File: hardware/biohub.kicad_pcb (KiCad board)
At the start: 4 copper layers, 89 x 55 mm, 123 parts, among them J1 CONNECTOR, J2 Conn_02x13_Odd_Even, U1 VAL**, U10 RM_10, U11 RM_10, U12 DCK6, U13 DCK6, U2 MCP2210-I_SS, U3 RI_16_1, U4 R_8, U5 ADP7142AUJZ-2.5-R7, U6 ADP7182AUJZ-2.5-R7, U7 VAL**, U8 RM_10, U9 RM_10

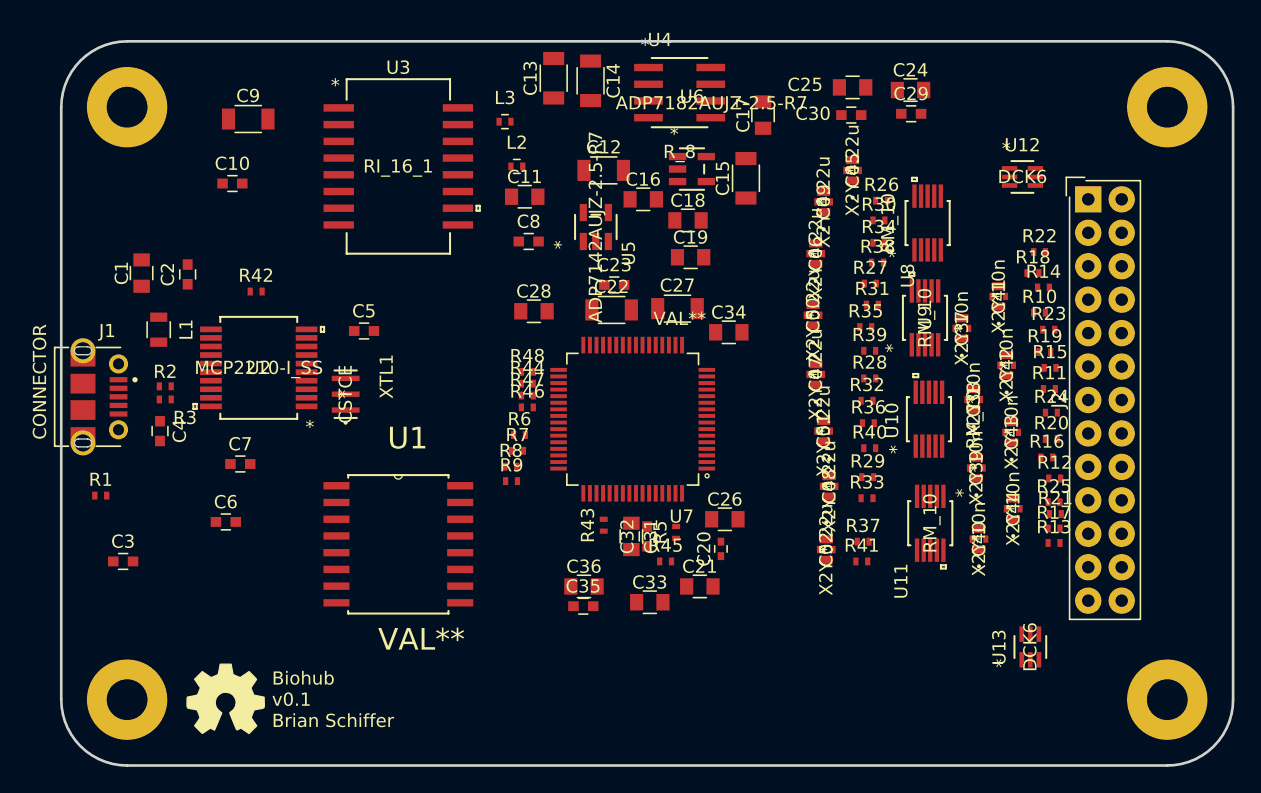
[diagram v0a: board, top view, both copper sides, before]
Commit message: Placement cleanup
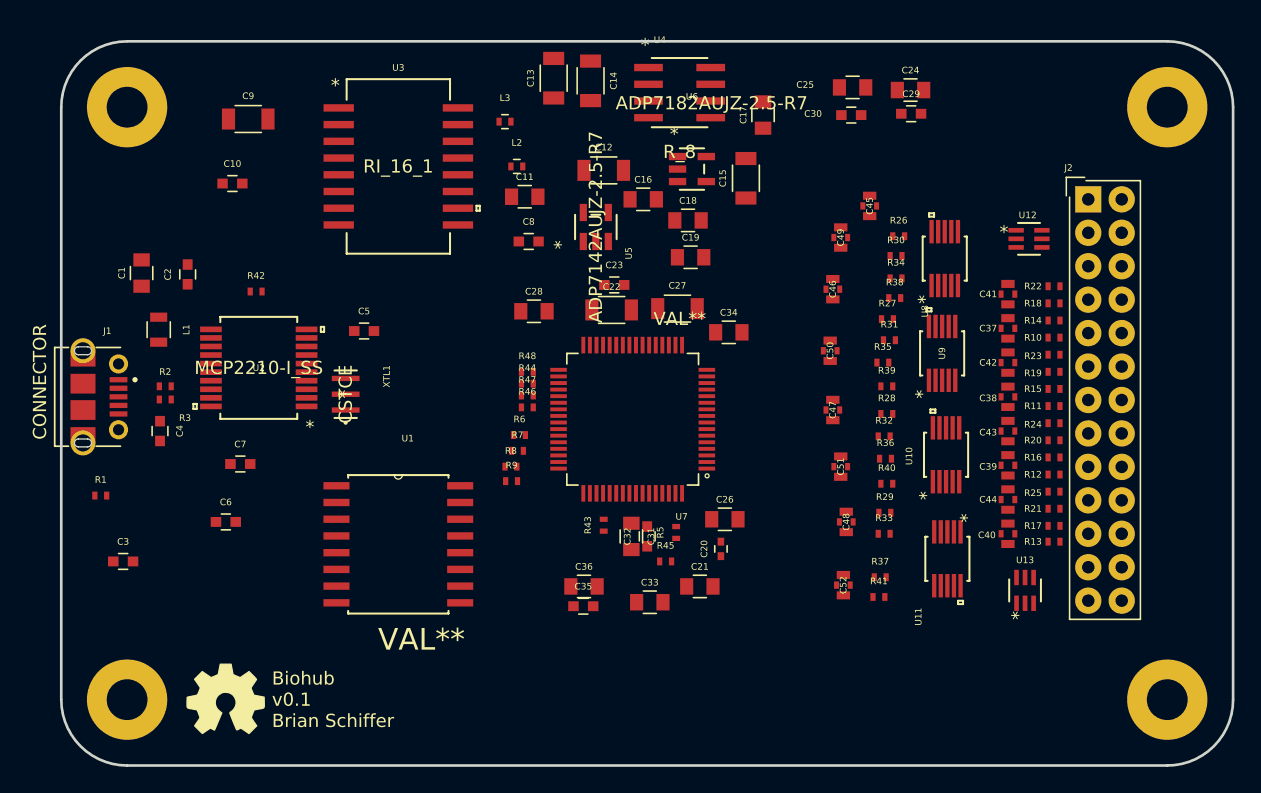
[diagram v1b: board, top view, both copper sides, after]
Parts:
- moved U12 4.73 mm to (178.0, 80.0)
- moved U13 4.32 mm to (177.7, 106.7)
- moved C37 3.50 mm to (176.4, 86.8)
- moved C45 3.00 mm to (165.9, 77.5)
- moved C48 3.00 mm to (164.1, 101.5)
- moved C50 3.00 mm to (162.9, 88.5)
- moved C52 3.00 mm to (163.9, 106.3)
- moved R29 3.00 mm to (167.1, 100.8)
- moved R30 3.00 mm to (167.9, 81.3)
- moved R31 3.00 mm to (167.4, 87.7)
- moved R32 3.00 mm to (167.0, 95.0)
- moved R33 3.00 mm to (167.0, 102.4)
- moved R34 3.00 mm to (167.9, 83.0)
- moved R35 3.00 mm to (166.9, 89.4)
- moved R38 3.00 mm to (167.8, 84.5)
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
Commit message: Near final placement
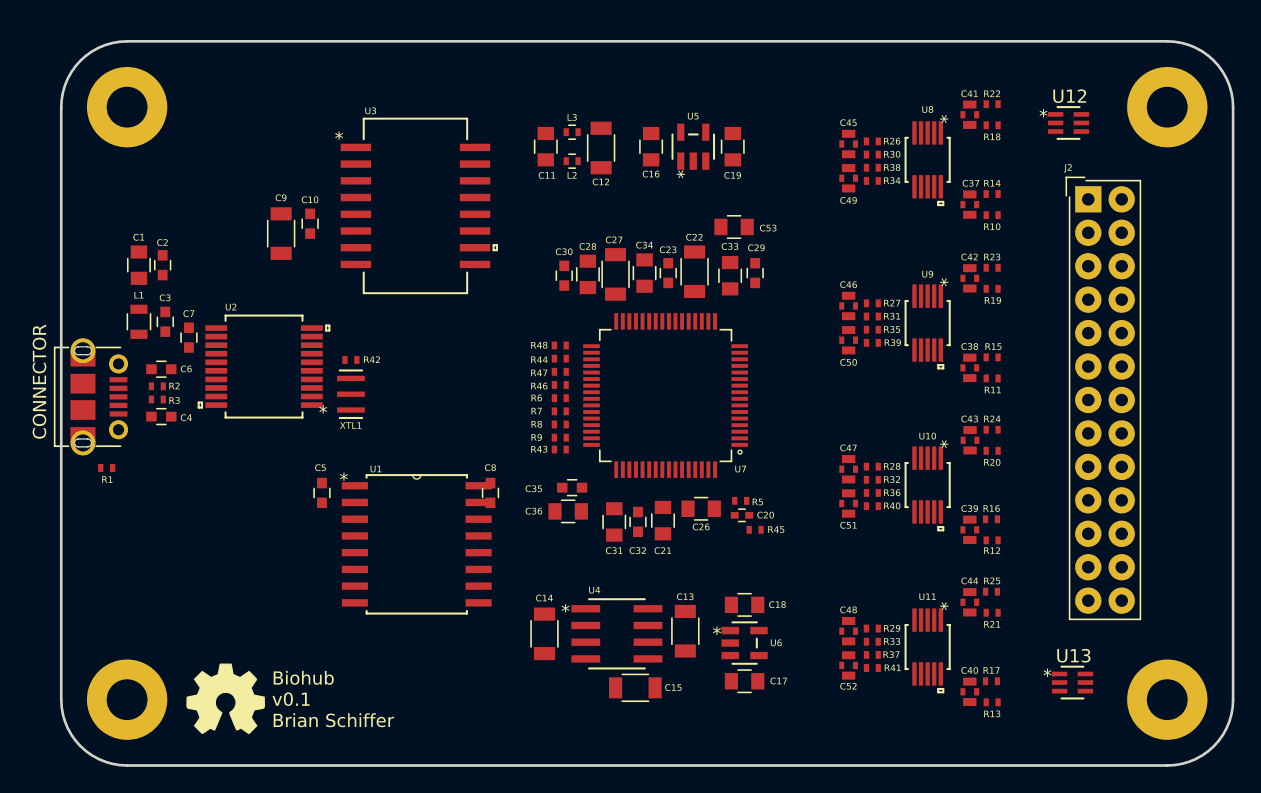
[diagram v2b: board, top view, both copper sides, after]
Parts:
- removed C24, C25: 1u, Capacitors_SMD:C_0805
- added C53: 1u, Capacitors_SMD:C_0805, F.Cu at (155.6, 79.1)
- U1: value VAL** -> **
- U7: value VAL** -> ADS1299
- moved C13 43.2 mm to (151.9, 109.8), turned to 270 degrees
- moved C17 43.0 mm to (156.4, 113.6), turned to 0 degrees
- moved C14 42.1 mm to (141.2, 110.0)
- moved U4 41.4 mm to (146.7, 110.0)
- moved C15 39.6 mm to (148.1, 114.1), turned to 180 degrees
- moved U6 36.2 mm to (156.4, 110.7)
- moved C18 29.5 mm to (156.4, 107.8), turned to 180 degrees
- moved C33 25.5 mm to (155.3, 82.8), turned to 270 degrees
- moved C30 25.0 mm to (142.7, 82.8), turned to 270 degrees
- moved C8 19.3 mm to (137.1, 99.3), turned to 270 degrees
- moved C3 18.5 mm to (112.4, 86.3), turned to 90 degrees
- moved C29 16.9 mm to (157.2, 82.6), turned to 270 degrees
- moved R22 14.6 mm to (175.2, 69.8)
- moved R18 14.3 mm to (175.2, 71.4)
- moved C41 13.9 mm to (173.5, 70.6)
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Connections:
- C49 pad 2: /interface/1N -> /interface/2N
- C51 pad 2: /interface/6P -> /interface/6N
- U12 pad 2: /AFE/BIAS -> Net-(U12-Pad2)
- U12 pad 4: Net-(U12-Pad4) -> /AFE/BIAS
- U13 pad 1: -2V5 -> /AFE/SRB2
- U13 pad 2: /AFE/SRB1 -> Net-(U13-Pad2)
- U13 pad 4: /AFE/SRB2 -> -2V5
- U13 pad 5: Net-(U13-Pad5) -> /AFE/SRB1
